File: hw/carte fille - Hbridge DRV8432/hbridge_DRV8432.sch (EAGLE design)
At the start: 41 parts, among them IC1 DRV8402, X4 M1-2, X5 M3-4, X6 +12V, X7 +24V

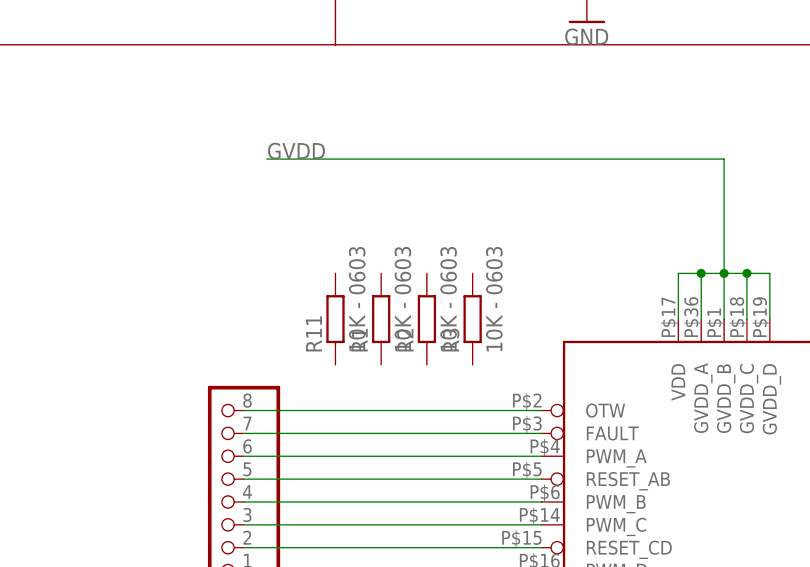
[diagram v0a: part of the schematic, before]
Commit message: finish routing
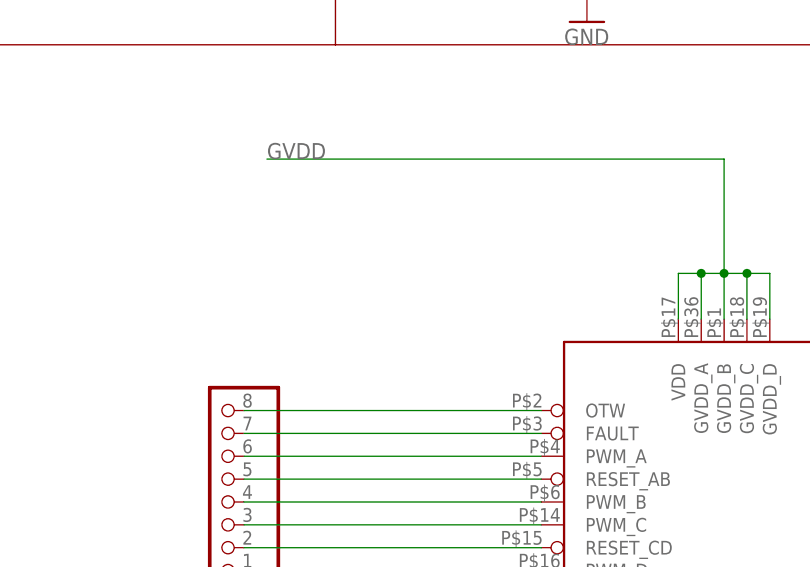
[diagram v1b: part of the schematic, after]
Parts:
- removed R1, R11, R2, R3: 10K - 0603, resistor:R-EU_R0603
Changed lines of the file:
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@@
 <part name="GND4" library="supply1" deviceset="GND" device=""/>
 <part name="GND6" library="supply1" deviceset="GND" device=""/>
-<part name="R11" library="resistor" deviceset="R-EU_" device="R0603" value="10K - 0603"/>
-<part name="R1" library="resistor" deviceset="R-EU_" device="R0603" value="10K - 0603"/>
-<part name="R2" library="resistor" deviceset="R-EU_" device="R0603" value="10K - 0603"/>
-<part name="R3" library="resistor" deviceset="R-EU_" device="R0603" value="10K - 0603"/>
 <part name="R4" library="resistor" deviceset="R-EU_" device="R0603" value="0R"/>
 <part name="R7" library="resistor" deviceset="R-EU_" device="R0603" value="0R"/>
@@
 <instance part="GND4" gate="1" x="-66.04" y="71.12"/>
 <instance part="GND6" gate="1" x="-15.24" y="60.96"/>
-<instance part="R11" gate="G$1" x="-43.18" y="27.94" rot="R90"/>
-<instance part="R1" gate="G$1" x="-38.1" y="27.94" rot="R90"/>
-<instance part="R2" gate="G$1" x="-33.02" y="27.94" rot="R90"/>
-<instance part="R3" gate="G$1" x="-27.94" y="27.94" rot="R90"/>
 <instance part="R4" gate="G$1" x="-30.48" y="-10.16" rot="R180"/>
 <instance part="R7" gate="G$1" x="-30.48" y="-12.7" rot="R180"/>
